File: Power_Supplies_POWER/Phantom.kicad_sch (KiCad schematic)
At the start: 19 parts, among them IC1 NCP731ADNADJR2G, IC2 LT8338

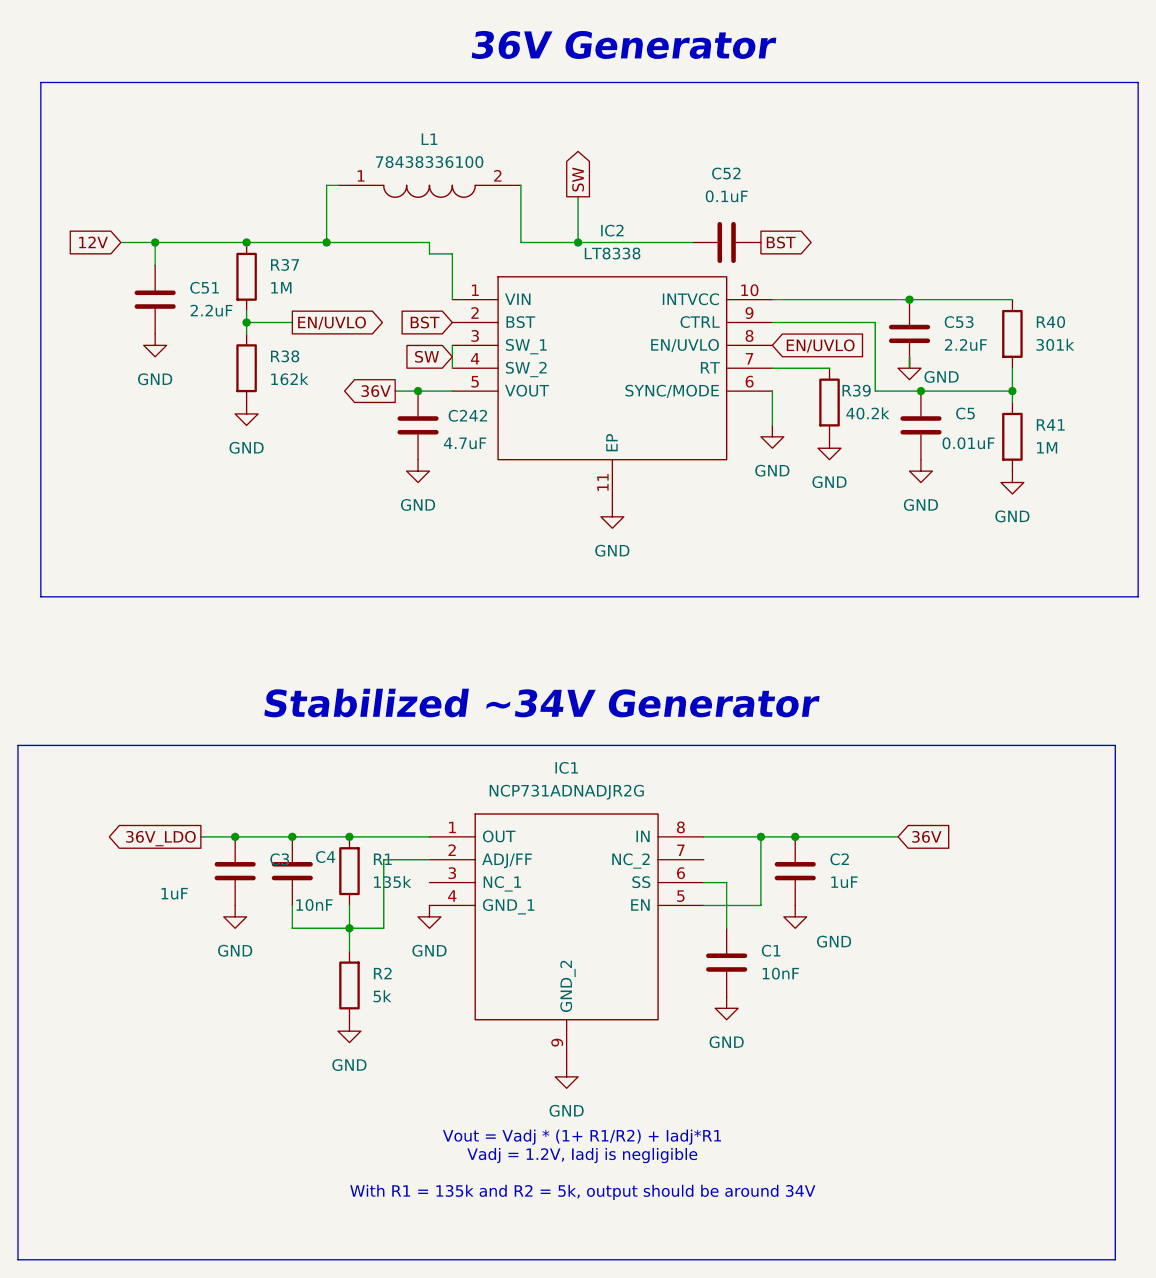
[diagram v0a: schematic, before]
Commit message: aaaah (cooked)
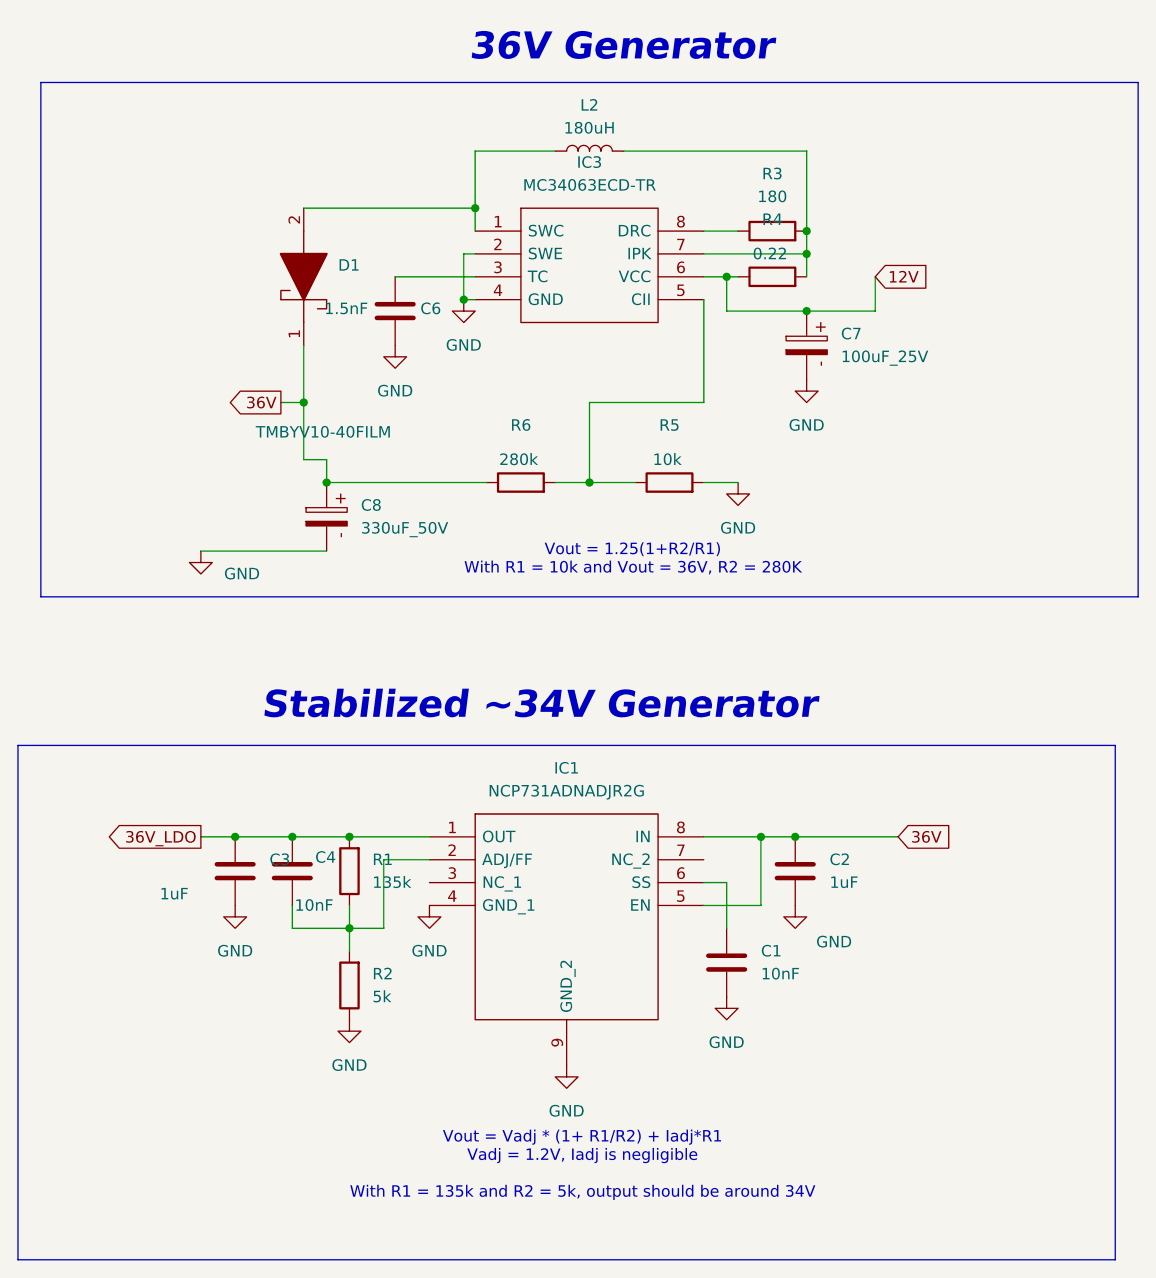
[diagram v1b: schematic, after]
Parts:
- removed C242: 4.7uF, Capacitor_SMD:C_0805_2012Metric_Pad1.18x1.45mm_HandSolder, symbol Device:C
- removed C5: 0.01uF, Capacitor_SMD:C_0402_1005Metric_Pad0.74x0.62mm_HandSolder, symbol Device:C
- removed C51, C53: 2.2uF, Capacitor_SMD:C_0805_2012Metric_Pad1.18x1.45mm_HandSolder, symbol Device:C
- removed C52: 0.1uF, Capacitor_SMD:C_0402_1005Metric, symbol Device:C
- removed IC2: LT8338, SamacSys_Parts:SOP50P490X110-11N, symbol SamacSys_Parts:lt8338
- removed L1: 78438336100, SamacSys_Parts:INDC3030X200N, symbol SamacSys_Parts:78438336100
- removed R37, R41: 1M, PCM_Resistor_SMD_AKL:R_0402_1005Metric_Pad0.72x0.64mm_HandSolder, symbol Device:R
- removed R38: 162k, PCM_Resistor_SMD_AKL:R_0402_1005Metric_Pad0.72x0.64mm_HandSolder, symbol Device:R
- removed R39: 40.2k, PCM_Resistor_SMD_AKL:R_0402_1005Metric_Pad0.72x0.64mm_HandSolder, symbol Device:R
- removed R40: 301k, PCM_Resistor_SMD_AKL:R_0402_1005Metric_Pad0.72x0.64mm_HandSolder, symbol Device:R
- added C6: 1.5nF, Capacitor_SMD:C_0805_2012Metric_Pad1.18x1.45mm_HandSolder, symbol Device:C
- added C7: 100uF_25V, Capacitor_SMD:CP_Elec_6.3x5.4, symbol PCM_SL_Capacitors:100uF_50V
- added C8: 330uF_50V, Capacitor_SMD:CP_Elec_10x10.5, symbol PCM_SL_Capacitors:220uF_50V
- added D1: TMBYV10-40FILM, SamacSys_Parts:TMBYV1040FILM, symbol SamacSys_Parts:TMBYV10-40FILM
- added IC3: MC34063ECD-TR, SamacSys_Parts:SOIC127P600X175-8N, symbol SamacSys_Parts:MC34063ECD-TR
- added L2: 180uH, Inductor_SMD:L_Vishay_IHLP-1212, symbol Device:L
- added R3: 180, PCM_Resistor_SMD_AKL:R_0805_2012Metric_Pad1.15x1.40mm_HandSolder, symbol Device:R
- added R4: 0.22, PCM_Resistor_SMD_AKL:R_2512_6332Metric_Pad1.40x3.35mm_HandSolder, symbol Device:R
- added R5: 10k, PCM_Resistor_SMD_AKL:R_0805_2012Metric_Pad1.15x1.40mm_HandSolder, symbol Device:R
- added R6: 280k, PCM_Resistor_SMD_AKL:R_0805_2012Metric_Pad1.15x1.40mm_HandSolder, symbol Device:R
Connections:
- net 12V: now also C7.1, IC3.6 (VCC), R4.1
- net 36V: now also C8.1, D1.1, R6.1
- net GND: now also C6.2, C7.2, C8.2, IC3.2 (SWE), IC3.4 (GND), R5.2
- new net: IC3.5 (CII), R5.1, R6.2
- new net: C6.1, IC3.3 (TC)
- new net: D1.2, IC3.1 (SWC), L2.1
- new net: IC3.7 (IPK), L2.2, R3.2, R4.2
- new net: IC3.8 (DRC), R3.1
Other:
- note added: "Vout = 1.25(1+R2/R1) With R1 = 10k and Vout = 36V, R2 = 280K"
